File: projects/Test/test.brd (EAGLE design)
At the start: 63.5 x 24.1 mm, 47 parts, among them J2 1755529, U1 STM32F405RGT6, U2 CSD88584Q5DCT, U3 CSD88584Q5DCT, U4 CSD88584Q5DCT, Y1 ECS-80-S-4X

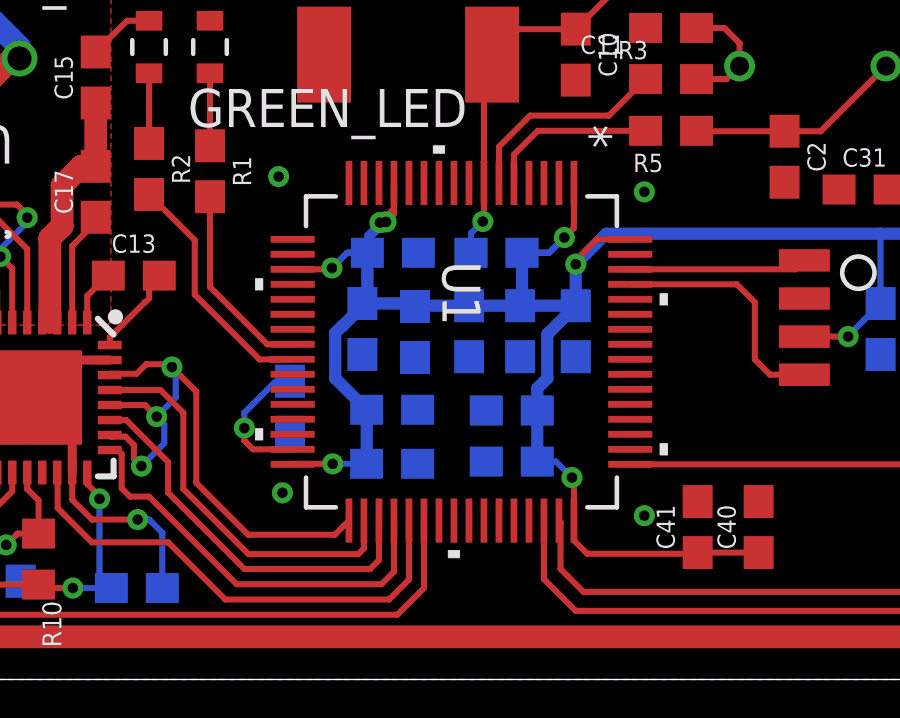
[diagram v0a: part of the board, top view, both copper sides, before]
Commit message: some stuff
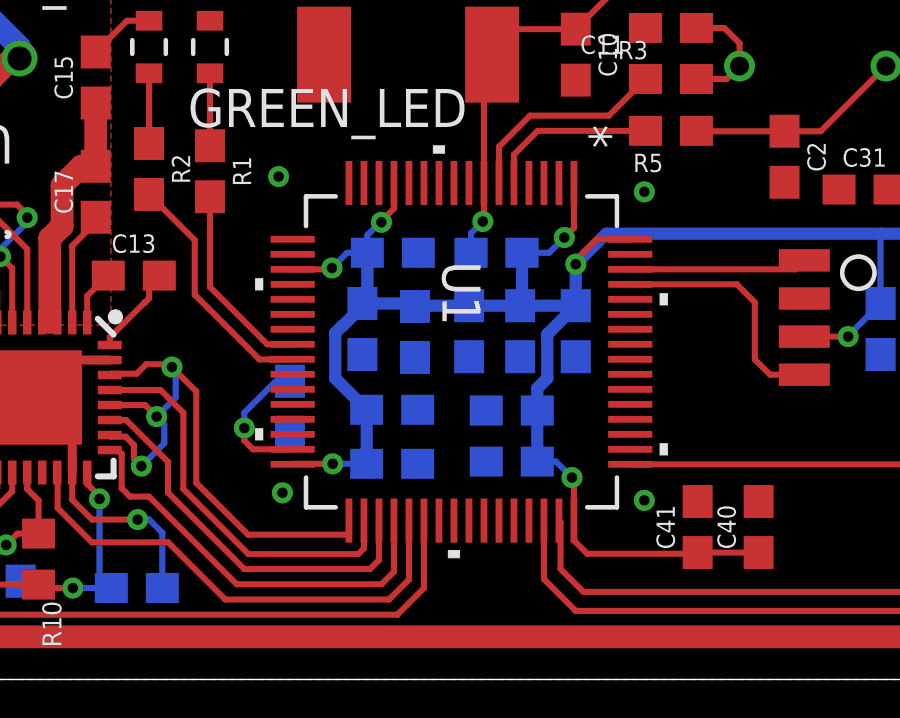
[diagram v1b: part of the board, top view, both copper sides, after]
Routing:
- net 3V3: track 76.5 -> 71.3 mm, vias 8 -> 7
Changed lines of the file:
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@@
 <via x="34.29" y="16.764" extent="1-16" drill="0.35"/>
 <via x="46.482" y="16.256" extent="1-16" drill="0.35"/>
-<via x="46.482" y="5.461" extent="1-16" drill="0.35"/>
+<via x="46.482" y="5.969" extent="1-16" drill="0.35"/>
 <via x="34.417" y="6.223" extent="1-16" drill="0.35"/>
 </signal>
@@
 <wire x1="44.136" y1="15.053" x2="43.815" y2="14.732" width="0.2032" layer="1"/>
 <via x="43.815" y="14.732" extent="1-16" drill="0.35"/>
-<via x="37.6682" y="15.2301" extent="1-16" drill="0.35"/>
-<wire x1="38.136" y1="16.5481" x2="38.136" y2="15.6979" width="0.2032" layer="1"/>
-<wire x1="38.136" y1="15.6979" x2="37.6682" y2="15.2301" width="0.2032" layer="1"/>
-<wire x1="43.815" y1="14.732" x2="43.307" y2="14.224" width="0.2032" layer="16"/>
-<wire x1="43.307" y1="14.224" x2="42.4044" y2="14.224" width="0.2032" layer="16"/>
+<wire x1="38.136" y1="15.6979" x2="38.136" y2="16.5481" width="0.2032" layer="1"/>
 <wire x1="37.25" y1="14.224" x2="37.25" y2="14.6341" width="0.2032" layer="16"/>
-<wire x1="37.25" y1="14.6341" x2="37.8714" y2="15.2555" width="0.2032" layer="16"/>
-<via x="37.8714" y="15.2555" extent="1-16" drill="0.35"/>
-<wire x1="38.136" y1="16.5481" x2="38.136" y2="15.5201" width="0.2032" layer="1"/>
-<wire x1="38.136" y1="15.5201" x2="37.8714" y2="15.2555" width="0.2032" layer="1"/>
-<wire x1="37.25" y1="14.224" x2="36.576" y2="14.224" width="0.2032" layer="16"/>
-<wire x1="36.576" y1="14.224" x2="36.068" y2="13.716" width="0.2032" layer="16"/>
 <via x="36.068" y="13.716" extent="1-16" drill="0.35"/>
 <wire x1="34.7599" y1="13.672" x2="36.024" y2="13.672" width="0.2032" layer="1"/>
@@
 <wire x1="40.64" y1="12.4578" x2="42.3418" y2="12.4578" width="0.4064" layer="16"/>
 <wire x1="42.3418" y1="12.4578" x2="42.3858" y2="12.4138" width="0.4064" layer="16"/>
-<wire x1="37.6682" y1="15.2301" x2="37.25" y2="14.8119" width="0.2032" layer="16"/>
-<wire x1="37.25" y1="14.8119" x2="37.25" y2="14.224" width="0.2032" layer="16"/>
+<wire x1="37.25" y1="14.224" x2="37.25" y2="14.8119" width="0.2032" layer="16"/>
 <wire x1="36.068" y1="13.716" x2="36.576" y2="14.224" width="0.2032" layer="16"/>
 <wire x1="36.576" y1="14.224" x2="37.25" y2="14.224" width="0.2032" layer="16"/>
@@
 <wire x1="43.815" y1="14.732" x2="43.307" y2="14.224" width="0.2032" layer="16"/>
 <wire x1="43.307" y1="14.224" x2="42.4044" y2="14.224" width="0.2032" layer="16"/>
+<wire x1="37.25" y1="14.8119" x2="37.6781" y2="15.24" width="0.2032" layer="16"/>
+<wire x1="37.6781" y1="15.24" x2="37.719" y2="15.24" width="0.2032" layer="16"/>
+<via x="37.719" y="15.24" extent="1-16" drill="0.35"/>
+<wire x1="37.719" y1="15.24" x2="37.719" y2="15.2809" width="0.2032" layer="1"/>
+<wire x1="37.719" y1="15.2809" x2="38.136" y2="15.6979" width="0.2032" layer="1"/>
 </signal>
 <signal name="N$5">
@@
 <contactref element="U$2" pad="28"/>
 <wire x1="31.5468" y1="6.5532" x2="33.274" y2="4.826" width="0.2032" layer="1"/>
-<wire x1="33.274" y1="4.826" x2="36.1661" y2="4.826" width="0.2032" layer="1"/>
-<wire x1="36.1661" y1="4.826" x2="36.636" y2="5.2959" width="0.2032" layer="1"/>
+<wire x1="33.274" y1="4.826" x2="36.5471" y2="4.826" width="0.2032" layer="1"/>
+<wire x1="36.636" y1="4.9149" x2="36.636" y2="5.2959" width="0.2032" layer="1"/>
+<wire x1="36.636" y1="4.9149" x2="36.5471" y2="4.826" width="0.2032" layer="1"/>
 <wire x1="28.662" y1="8.148" x2="28.7149" y2="8.0951" width="0.2032" layer="1"/>
 <wire x1="28.7149" y1="8.0951" x2="29.18825" y2="8.0951" width="0.2032" layer="1"/>
@@
 <mfgpreviewcolor name="substratecolor" color="0xFF786E46"/>
 </mfgpreviewcolors>
-<errors>
-</errors>
 </board>
 </drawing>
